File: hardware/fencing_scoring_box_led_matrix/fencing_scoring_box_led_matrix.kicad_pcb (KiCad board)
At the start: 2 copper layers, 100 x 70 mm, 11 parts, among them J2 Conn_01x05_Pin

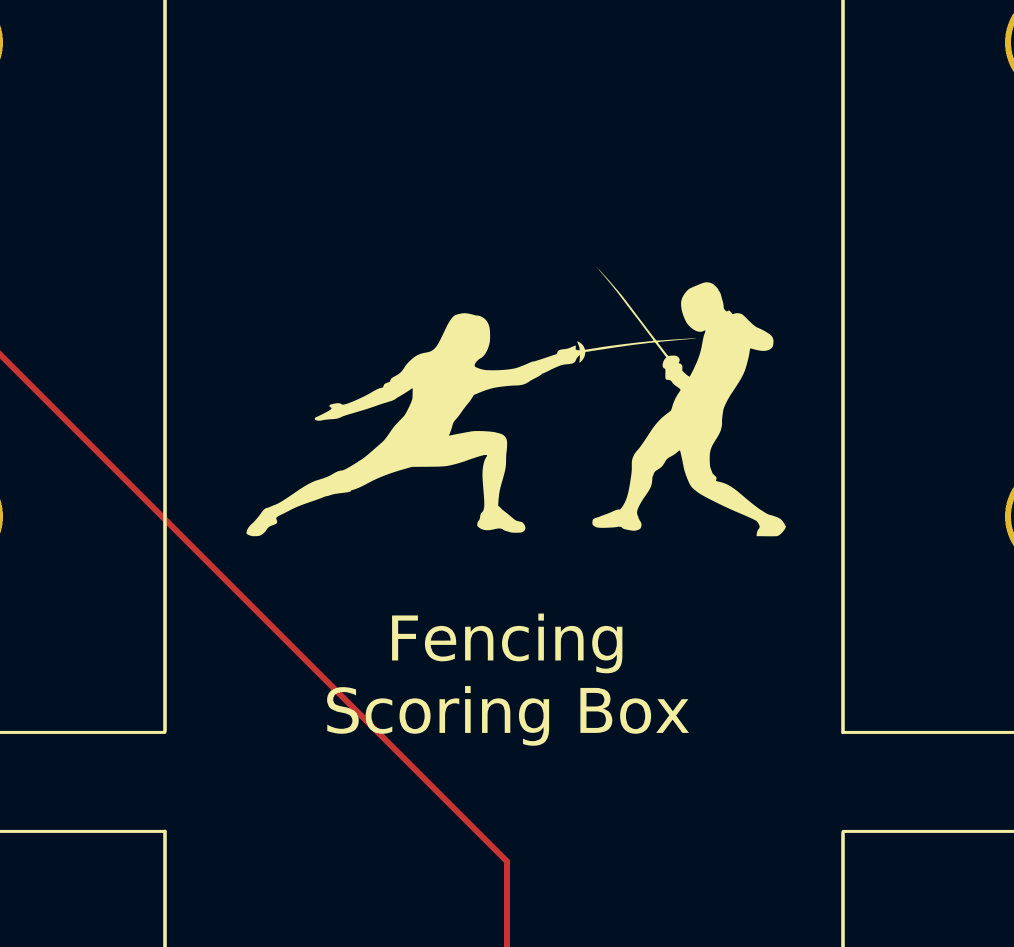
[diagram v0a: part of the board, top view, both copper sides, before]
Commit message: Pin changes to arduino code and renaming pcb design
Changed the pins to be compatibe with the new PCB design for an arduino
nano
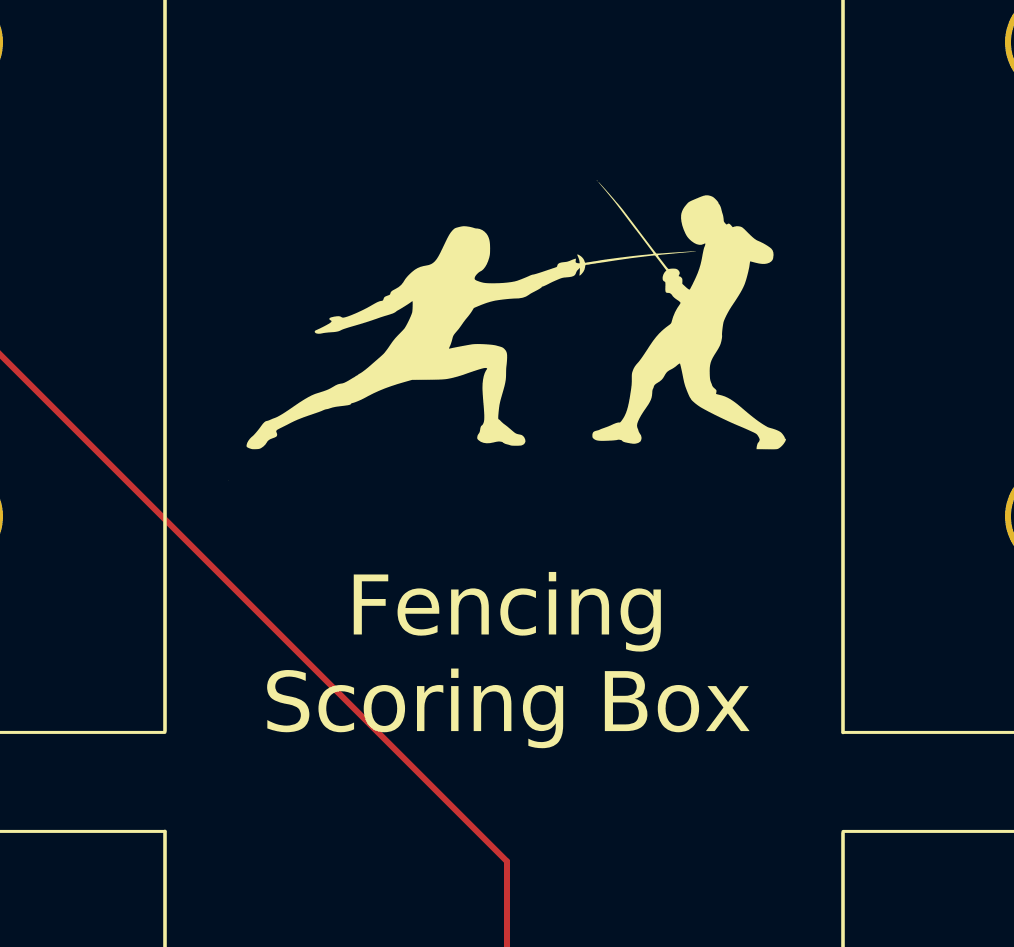
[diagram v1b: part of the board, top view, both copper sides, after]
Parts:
- moved G*** 2.90 mm to (150.6, 69.0)
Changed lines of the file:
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@@
 			(disableapertmacros no)
 			(usegerberextensions no)
-			(usegerberattributes yes)
-			(usegerberadvancedattributes yes)
-			(creategerberjobfile yes)
+			(usegerberattributes no)
+			(usegerberadvancedattributes no)
+			(creategerberjobfile no)
 			(dashed_line_dash_ratio 12.000000)
 			(dashed_line_gap_ratio 3.000000)
@@
 			(plotinvisibletext no)
 			(sketchpadsonfab no)
-			(subtractmaskfromsilk no)
+			(subtractmaskfromsilk yes)
 			(outputformat 1)
 			(mirror no)
@@
 	(footprint "Graphics:Fencers_20mm_h"
 		(layer "F.Cu")
-		(at 150.645168 71.899493)
+		(at 150.645168 69)
 		(property "Reference" "G***"
 			(at 0 0 0)
@@
 		(effects
 			(font
-				(size 1.5 1.5)
+				(size 2 2)
 				(thickness 0.15)
 			)
